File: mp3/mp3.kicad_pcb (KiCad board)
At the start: 2 copper layers, 33 parts, among them J1 USB4105-GF-A, J2 LEFT, J3 DEBUG, J4 RIGHT, U1 W25Q128JV, U2 RP2040, U3 MCP1702T-3302E_CB, Y1 12MHz

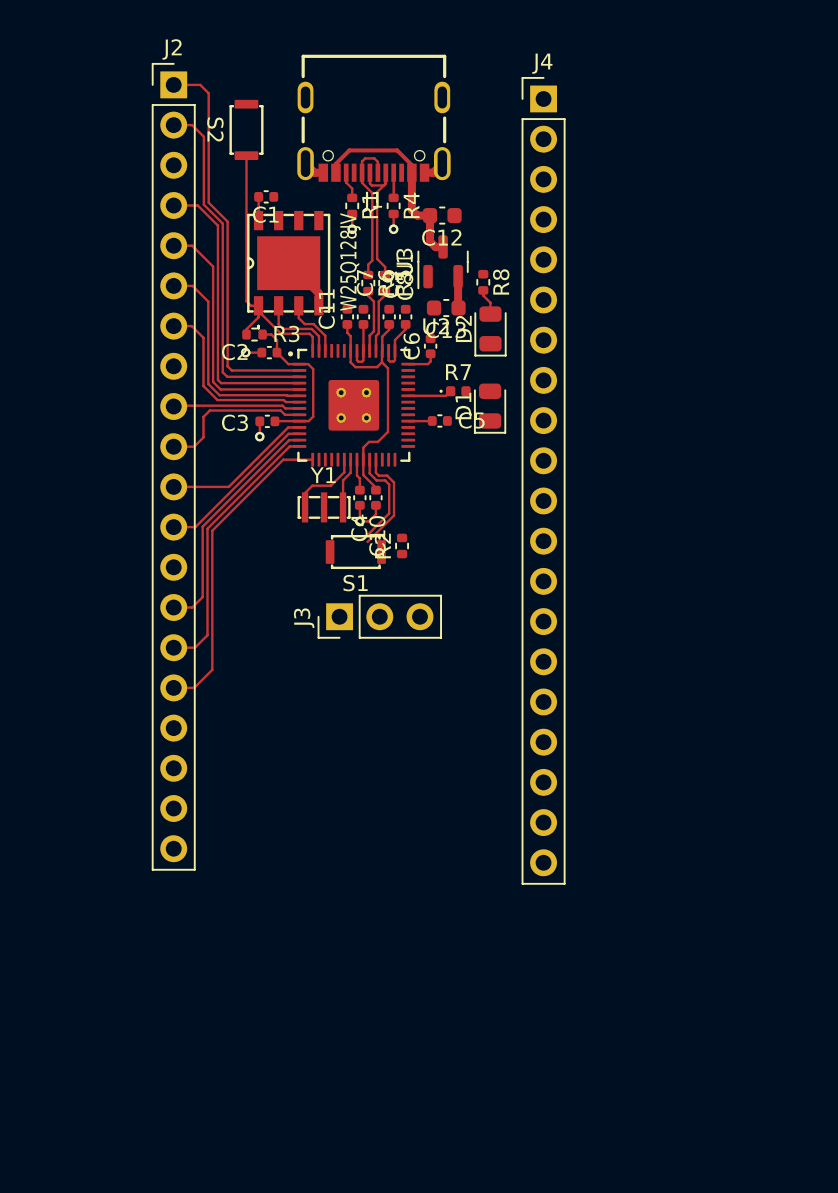
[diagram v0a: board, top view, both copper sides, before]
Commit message: completed mp3 layout
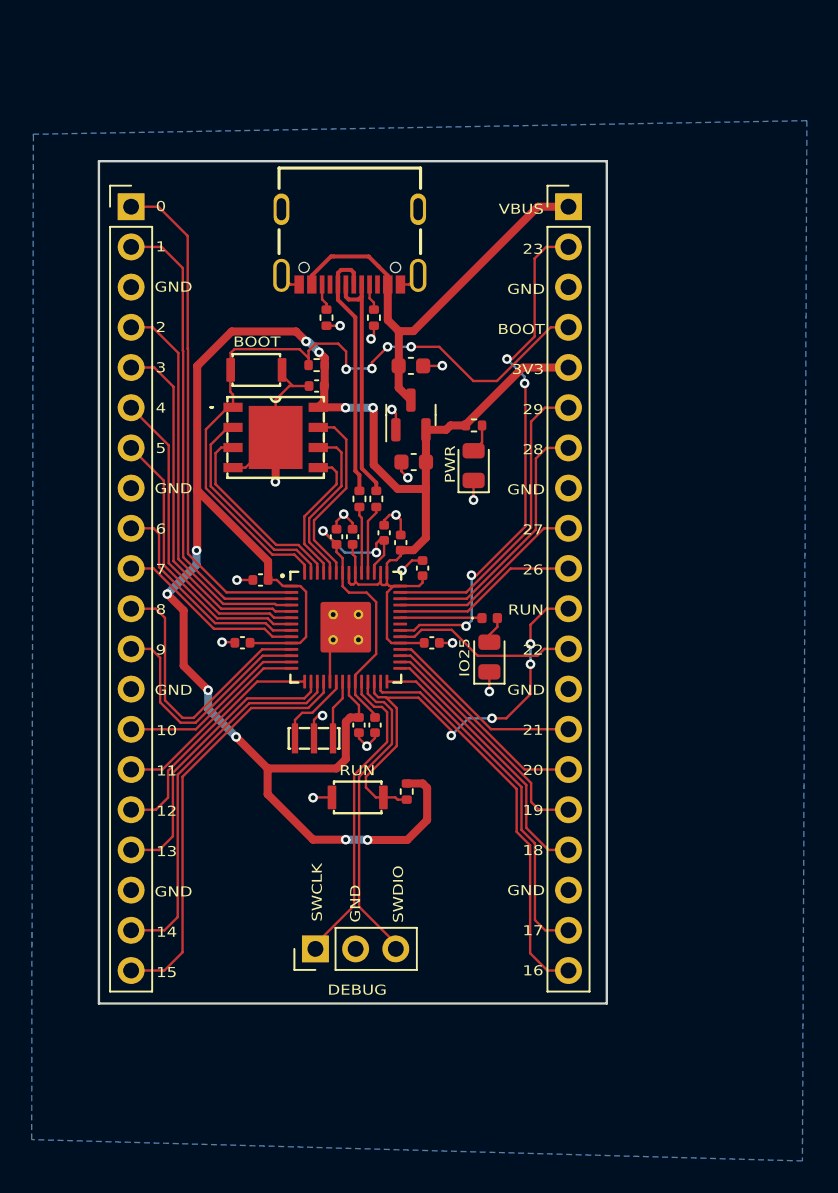
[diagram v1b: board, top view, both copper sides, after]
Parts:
- moved J3 21.0 mm to (156.7, 93.1)
- moved D1 15.9 mm to (167.7, 74.6)
- moved R2 15.5 mm to (162.5, 83.1)
- moved S1 15.5 mm to (159.4, 83.5)
- moved S2 15.2 mm to (153.0, 56.5), turned to 180 degrees
- moved Y1 14.6 mm to (156.6, 79.8)
- moved R7 14.5 mm to (167.7, 72.2)
- moved C2 14.4 mm to (153.3, 69.8)
- moved C10 14.4 mm to (160.5, 78.9)
- moved C4 14.4 mm to (159.5, 78.9)
- moved C8 14.3 mm to (162.1, 67.4)
- moved C3 14.1 mm to (152.1, 73.7)
- moved C5 14.0 mm to (164.1, 73.7)
- moved C6 14.0 mm to (163.5, 69.0)
- moved U2 14.0 mm to (158.6, 72.7)
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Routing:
- net +3V3: track 26.0 -> 135.3 mm, vias 0 -> 10
- net /GPIO23: track 0.00 -> 33.2 mm, vias 0 -> 4
- net /RUN: track 0.00 -> 29.8 mm, vias 0 -> 4
- net /BOOT: track 17.5 -> 45.5 mm, vias 0 -> 4
- net GND: track 12.9 -> 40.2 mm, vias 5 -> 17
- net /GPIO15: track 0.00 -> 26.6 mm
- net /GPIO16: track 0.00 -> 25.4 mm
- net /GPIO14: track 0.00 -> 23.9 mm
- net /GPIO17: track 0.00 -> 22.4 mm
- net /GPIO29: track 0.00 -> 19.4 mm
- net /GPIO13: track 0.00 -> 18.5 mm
- net /GPIO28: track 0.00 -> 17.2 mm
- net /GPIO18: track 0.00 -> 17.0 mm
- net /VBUS: track 12.8 -> 28.8 mm
- net /GPIO19: track 0.00 -> 15.2 mm
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- added copper zone on B.Cu, net GND
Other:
- board outline added: 32.1 x 53.2 mm
- board text added: "0"
- board text added: "1"
- board text added: "10"
- board text added: "11"
- board text added: "12"
- board text added: "13"
- board text added: "14"
- board text added: "15"
- board text added: "16"
- board text added: "17"
- board text added: "18"
- board text added: "19"
- board text added: "2"
- board text added: "20"
- board text added: "21"
- board text added: "22"
- board text added: "23"
- board text added: "26"
- board text added: "27"
- board text added: "28"
- board text added: "29"
- board text added: "3"
- board text added: "3V3"
- board text added: "4"
- board text added: "5"
- board text added: "6"
- board text added: "7"
- board text added: "8"
- board text added: "9"
- board text added: "BOOT"
- board text added: "DEBUG"
- board text added: "GND"
- board text added: "IO25"
- board text added: "PWR"
- board text added: "RUN"
- board text added: "SWCLK"
- board text added: "SWDIO"
- board text added: "VBUS"
